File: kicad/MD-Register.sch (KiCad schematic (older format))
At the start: 19 parts, among them U68 74LS245, U69 74LS173, U70 74LS173

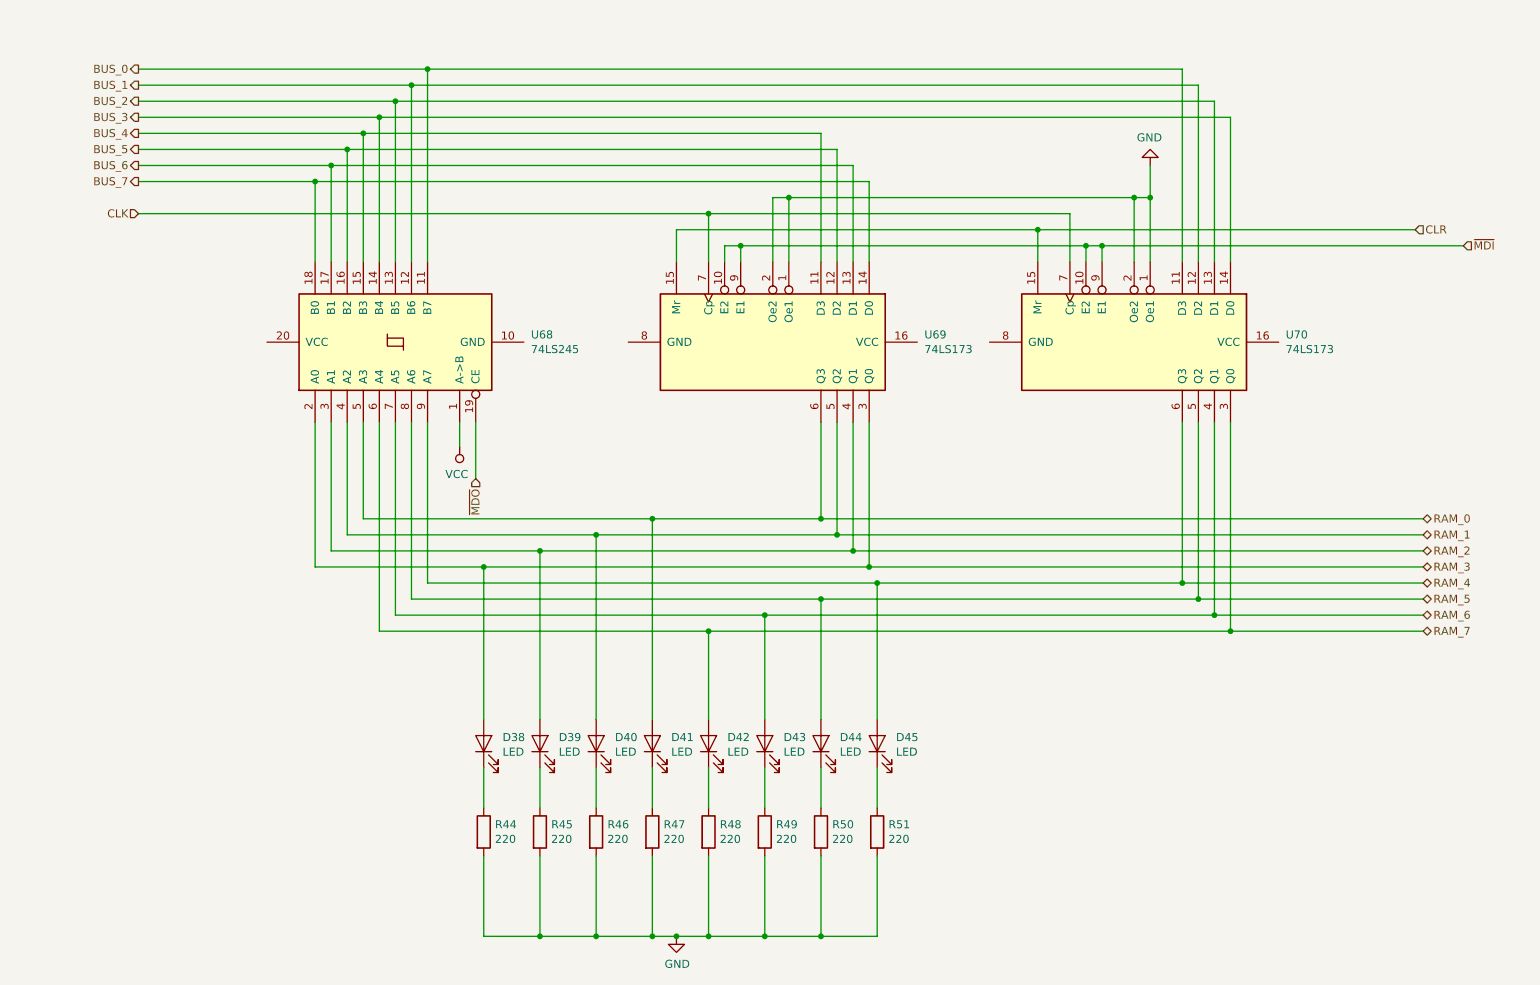
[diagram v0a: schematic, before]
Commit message: Up to v1.0 and plot
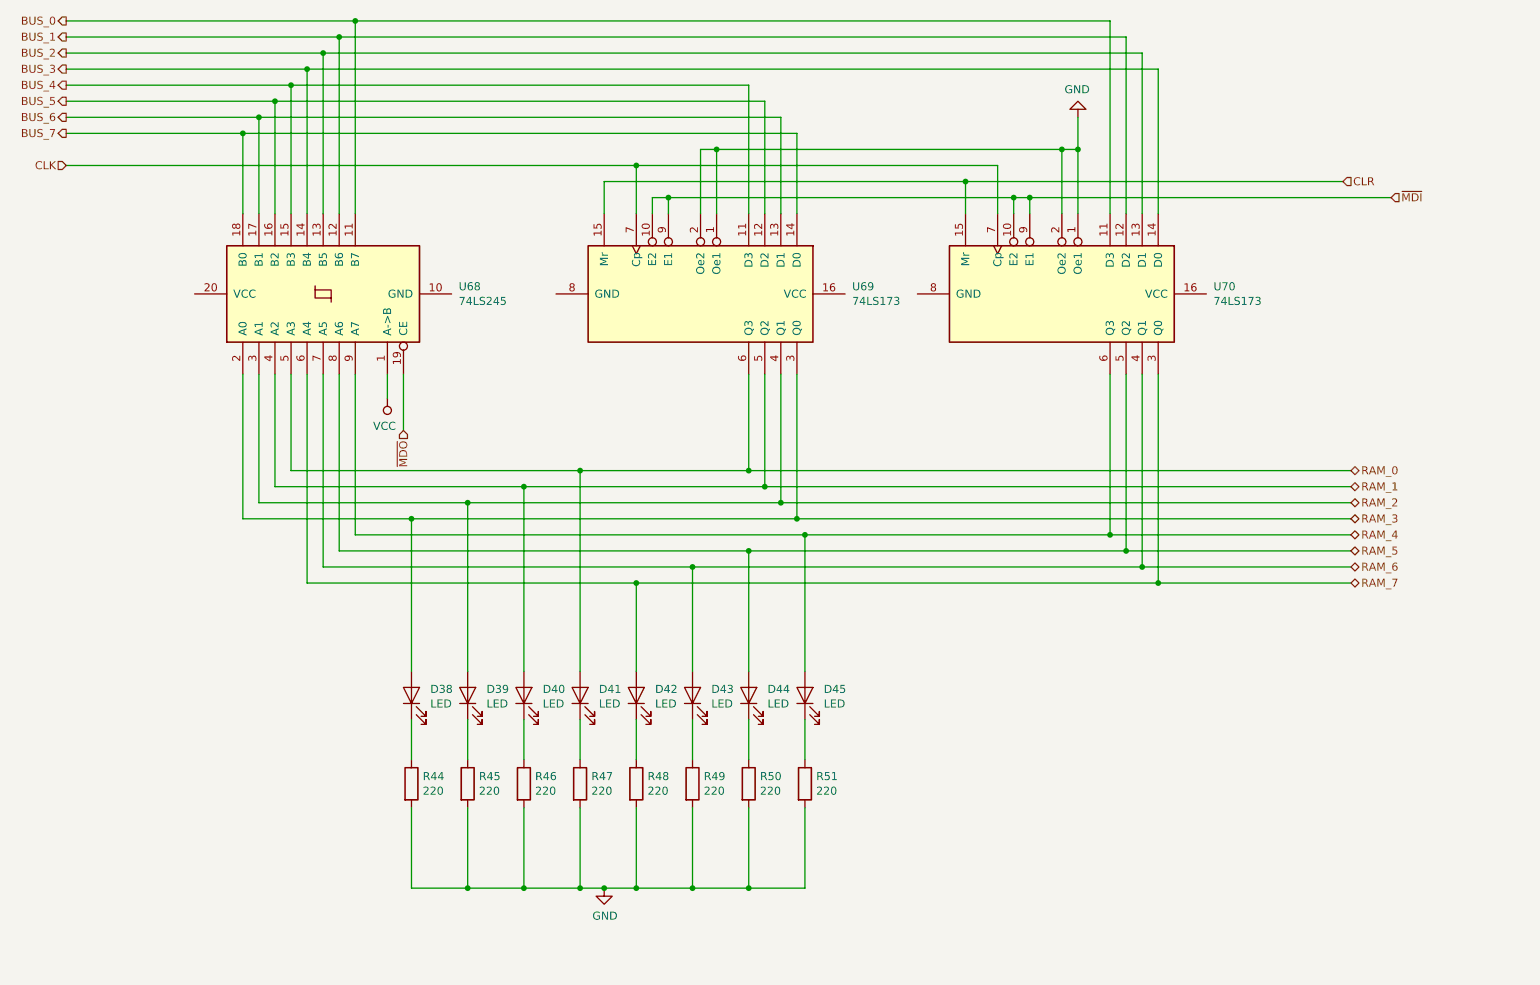
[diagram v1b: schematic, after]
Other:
- moved on the sheet: D38, D39, D40, D41, D42, D43, D44, D45, R44, R45, R46, R47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
